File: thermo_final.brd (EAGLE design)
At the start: 7.9 x 13.4 mm, 109 parts, among them IC1 DG4051EEQ-T1-GE3, IC2 DG4051EEQ-T1-GE3, IC5 MAX6675ISA+, T1 782482_33VC

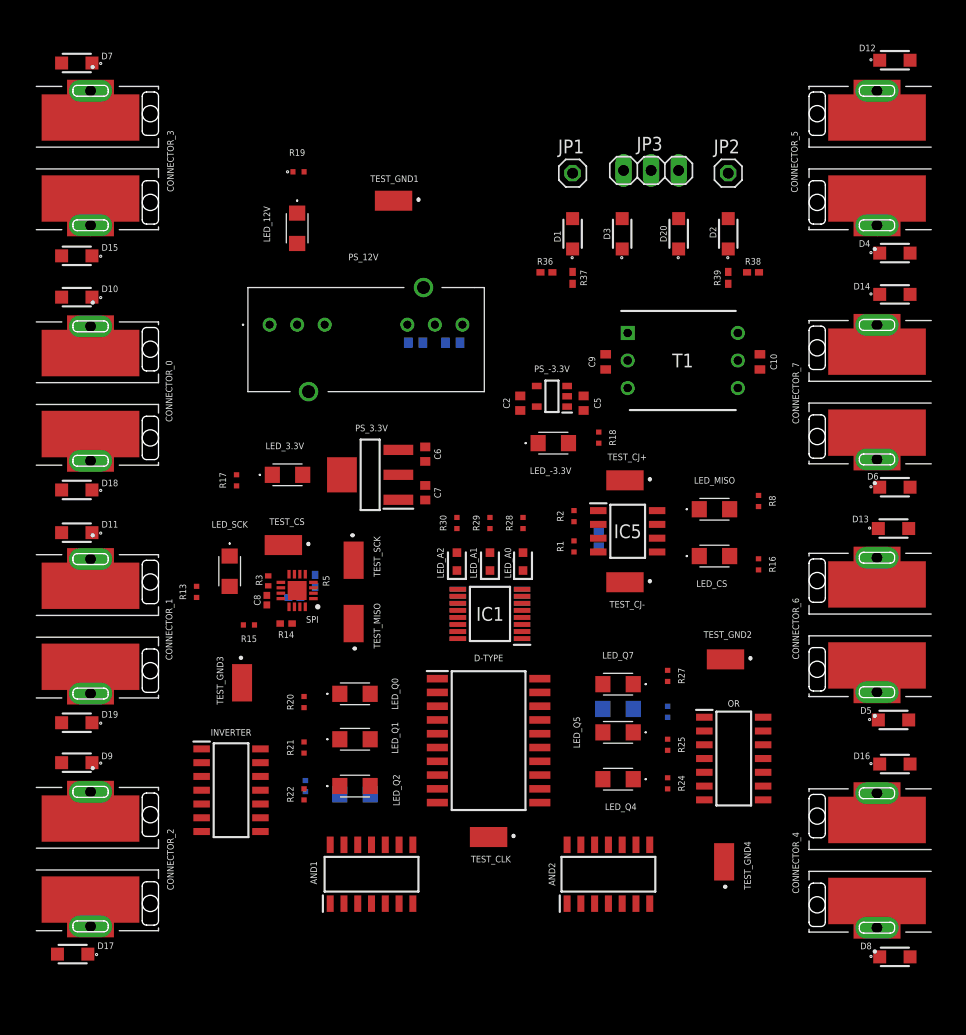
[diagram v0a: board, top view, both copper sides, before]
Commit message: routing save
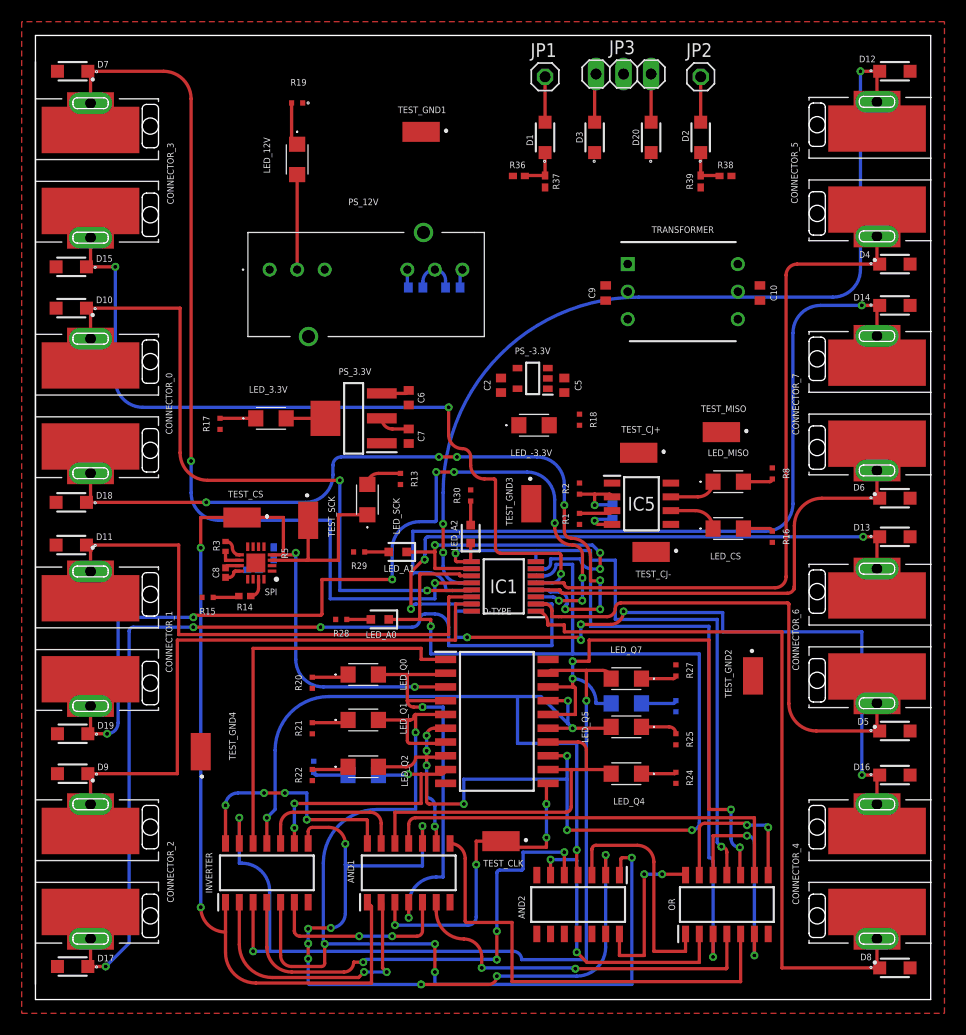
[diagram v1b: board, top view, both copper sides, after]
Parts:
- removed T1: 782482_33VC, SamacSys_Parts:DIP1016W60P254L914H635Q6N
- added TRANSFORMER: 782482_33VC, SamacSys_Parts:DIP1016W60P254L914H635Q6N
- moved TEST_GND4 49.3 mm to (38.1, 0.00)
- moved TEST_MISO 38.2 mm to (86.1, 29.5), turned to 0 degrees
- moved TEST_GND3 31.4 mm to (68.6, 22.9)
- moved R13 21.5 mm to (56.5, 25.1), turned to 90 degrees
- moved R28 19.0 mm to (51.1, 12.2), turned to 0 degrees
- moved LED_SCK 14.3 mm to (53.5, 23.2), turned to 90 degrees
- moved LED_A0 14.2 mm to (54.6, 12.2), turned to 180 degrees
- moved OR 13.5 mm to (86.6, -14.1), turned to 90 degrees
- moved R29 12.4 mm to (52.7, 18.4), turned to 0 degrees
- moved D1 9.25 mm to (69.8, 56.6)
- moved D2 9.25 mm to (84.2, 56.6)
- moved D3 9.25 mm to (74.4, 56.6)
- moved JP3 9.25 mm to (77.1, 62.5)
- moved R36 9.25 mm to (67.4, 53.1)
- moved R37 9.25 mm to (69.8, 52.6)
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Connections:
- net IM: now also TRANSFORMER.3; no longer T1.3
- net IMOUT: now also TRANSFORMER.4; no longer T1.4
- net IP: now also TRANSFORMER.1; no longer T1.1
- net IPOUT: now also TRANSFORMER.6; no longer T1.6
- net N$10: now also TRANSFORMER.2; no longer T1.2
- net N$14: now also TRANSFORMER.5; no longer T1.5
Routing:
- net Q3: track 0.00 -> 132.2 mm, vias 0 -> 8
- net CS: track 0.00 -> 113.1 mm, vias 0 -> 4
- net Q1: track 0.00 -> 96.5 mm, vias 0 -> 5
- net T3+: track 0.00 -> 85.6 mm, vias 0 -> 2
- net Q7: track 0.00 -> 84.5 mm, vias 0 -> 3
- net T2-: track 0.00 -> 83.3 mm, vias 0 -> 3
- net T1-: track 0.00 -> 83.3 mm, vias 0 -> 9
- net !Q7: track 0.00 -> 81.8 mm, vias 0 -> 4
- net A1: track 0.00 -> 81.3 mm, vias 0 -> 4
- net T5-: track 0.00 -> 80.0 mm, vias 0 -> 3
- net T7-: track 0.00 -> 73.9 mm, vias 0 -> 1
- net T3-: track 0.00 -> 73.7 mm, vias 0 -> 3
- net !Q3: track 0.00 -> 72.5 mm, vias 0 -> 9
- net Q5: track 0.00 -> 72.1 mm, vias 0 -> 4
- net T0-: track 0.00 -> 71.1 mm, vias 0 -> 7
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- added copper zone on layer 1, net GND
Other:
- board size 7.9 x 13.4 mm -> 82.5 x 88.9 mm
